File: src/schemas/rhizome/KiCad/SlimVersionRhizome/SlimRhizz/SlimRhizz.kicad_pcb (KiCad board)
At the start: 4 copper layers, 135 x 34.5 mm, 20 parts, among them J1 POWER_IN, J2 WS2812_Tip1, J3 WS2812_Tip2, J4 LED_TUBE, J5 Haptic_DRV1, J6 Haptic_DRV2, J7 Pogo_Male, J8 Pogo_Female, U2 74AHCT125

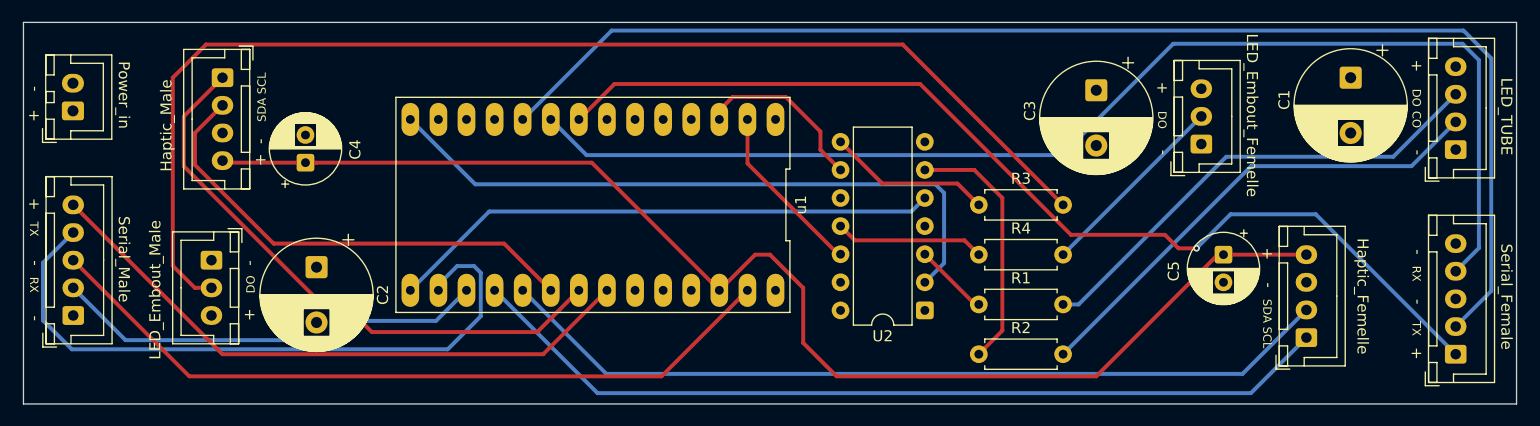
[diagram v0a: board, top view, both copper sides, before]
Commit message: pcb v2
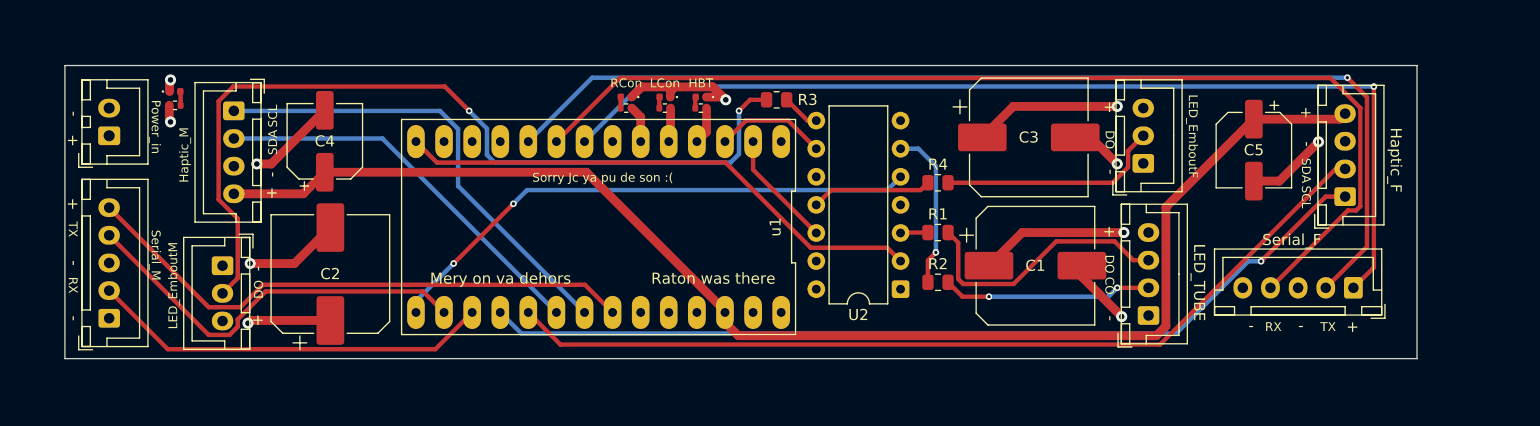
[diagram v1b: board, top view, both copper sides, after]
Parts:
- added D1: PWR, LED_SMD:LED_0402_1005Metric, F.Cu at (71.2, 113.2)
- added HBT: HBT, LED_SMD:LED_0402_1005Metric, F.Cu at (118.8, 113.8)
- added LCon: L-Connect, LED_SMD:LED_0402_1005Metric, F.Cu at (115.5, 113.8)
- added PWR: 1000, Resistor_SMD:R_0402_1005Metric, F.Cu at (71.2, 114.5)
- added R6: 330, Resistor_SMD:R_0402_1005Metric, F.Cu at (118.8, 114.8)
- added R7: 330, Resistor_SMD:R_0402_1005Metric, F.Cu at (115.5, 114.8)
- added R8: 330, Resistor_SMD:R_0402_1005Metric, F.Cu at (112.0, 114.8)
- added RCon: R-Connect, LED_SMD:LED_0402_1005Metric, F.Cu at (112.0, 113.8)
- C1, C2, C3: footprint Capacitor_THT:CP_Radial_D10.0mm_P5.00mm -> Capacitor_SMD:CP_Elec_10x10.5
- C4, C5: footprint Capacitor_THT:CP_Radial_D6.3mm_P2.50mm -> Capacitor_SMD:CP_Elec_6.3x5.4
- J4: value LED_TUBE -> APA102_Strip
- R1, R2, R4: footprint Resistor_THT:R_Axial_DIN0207_L6.3mm_D2.5mm_P7.62mm_Horizontal -> Resistor_SMD:R_0805_2012Metric
- R3: value 330 -> 220; footprint Resistor_THT:R_Axial_DIN0207_L6.3mm_D2.5mm_P7.62mm_Horizontal -> Resistor_SMD:R_0805_2012Metric
- moved C1 33.2 mm to (149.0, 129.0), turned to 0 degrees
- moved J4 31.6 mm to (159.2, 133.5)
- moved R3 20.6 mm to (125.6, 114.0), turned to 180 degrees
- moved J6 13.2 mm to (177.0, 122.8)
- moved J8 11.0 mm to (177.8, 131.0), turned to 180 degrees
- moved C5 9.84 mm to (168.8, 118.5)
- moved G*** 9.69 mm to (109.9, 125.1)
- moved R1 7.47 mm to (140.2, 126.0)
- moved R2 7.47 mm to (140.2, 130.5)
- moved R4 7.47 mm to (140.2, 121.5)
- moved C3 7.44 mm to (148.4, 117.4), turned to 0 degrees
- moved J3 5.53 mm to (158.8, 119.8)
- moved J1 3.97 mm to (65.2, 117.2)
- moved J7 3.26 mm to (65.2, 133.8)
- moved J5 3.17 mm to (76.5, 115.0)
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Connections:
- u1 pad 2: unconnected-(u1-Pad2) -> Net-(R6-Pad1)
- u1 pad 3: unconnected-(u1-Pad3) -> Net-(R7-Pad1)
- u1 pad 4: unconnected-(u1-Pad4) -> Net-(R8-Pad1)
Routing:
- net +5V: track 2.82 -> 35.9 mm, vias 0 -> 4
- net Net-(J2-Pin_2): track 109.1 -> 77.6 mm, vias 0 -> 2
- net GND: track 75.4 -> 48.4 mm, vias 0 -> 7
- net Net-(J4-Pin_2): track 44.2 -> 19.0 mm, vias 0 -> 2
- net Net-(J7-Pin_4): track 60.2 -> 36.8 mm
- net Net-(J8-Pin_2): track 117.5 -> 97.7 mm, vias 0 -> 1
- net Net-(J4-Pin_3): track 43.4 -> 24.3 mm
- net Net-(J8-Pin_4): track 110.0 -> 96.3 mm
- net /APA_CLK_PRE: track 59.8 -> 48.3 mm
- net Net-(R3-Pad1): track 14.9 -> 3.45 mm
- net Net-(J5-Pin_1): track 53.0 -> 42.3 mm
- net Net-(R2-Pad1): track 23.1 -> 14.6 mm, vias 0 -> 1
- net Net-(J5-Pin_2): track 43.3 -> 35.7 mm
- net Net-(J5-Pin_4): track 116.2 -> 122.6 mm
- net /LED_TIP1: track 16.0 -> 10.1 mm
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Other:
- board size 135 x 34.5 mm -> 122.2 x 26.5 mm
- board text added: "Big shoutout à la Cohorte de feu"
- board text added: "Haptic_F"
- board text added: "Haptic_M"
- board text added: "LED_EmboutF"
- board text added: "LED_EmboutM"
- board text added: "Mery on va dehors"
- board text added: "PCB DESIGN: Clément Boucher Justin Lepitre"
- board text added: "Raton was there"
- board text added: "Serial_F"
- board text added: "Serial_M"
- board text added: "Sorry Jc ya pu de son :("
- board text added: "Version 2.0"
- board text removed: "Haptic_Femelle"
- board text removed: "Haptic_Male"
- board text removed: "LED_Embout_Femelle"
- board text removed: "LED_Embout_Male"
- board text removed: "Serial_Female"
- board text removed: "Serial_Male"
